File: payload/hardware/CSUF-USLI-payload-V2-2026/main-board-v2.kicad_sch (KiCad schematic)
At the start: 29 parts, among them J1 Servo JST, J10 8.4V IN, J11 Chassis Input, J12 Servo VCC, J13 Servo GND, J14 11.1V IN, J15 8.4V RESERVE, J16 11.1V RESERVE, J17 Driver Input, J2 Drill x 11.1V OUT, J4 BTS7960 Output, J6 Reserve JST, J9 Soil Sensor Power, Q3 IRLZ44N, U1 DEV-16771, U2 Adafruit BMP280, U3 RYLR896, U4 RYLR896, U5 Modbus to UART

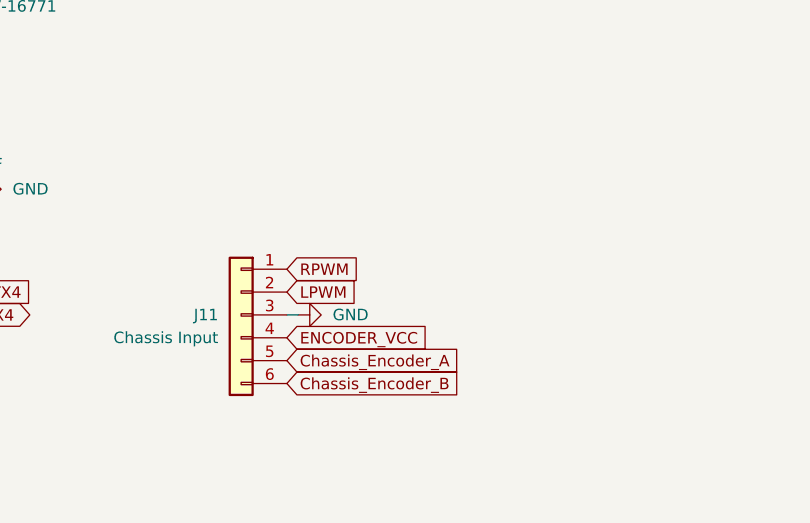
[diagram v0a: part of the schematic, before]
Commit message: trying to route traces
bad bad bad
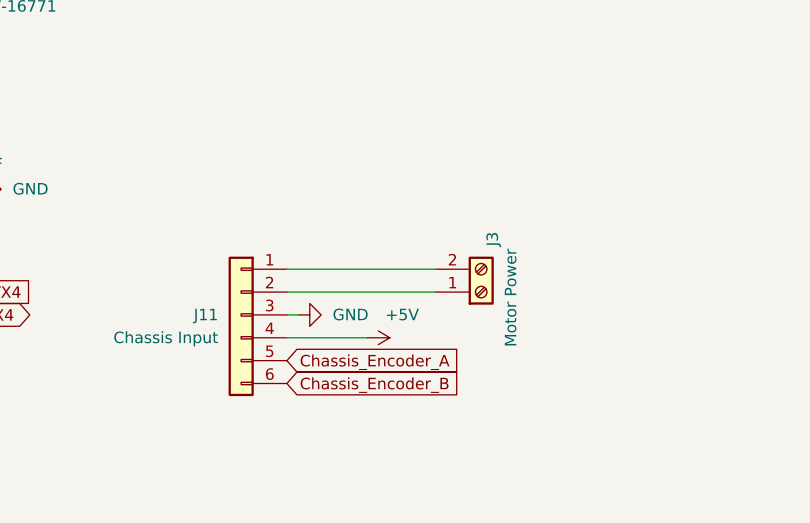
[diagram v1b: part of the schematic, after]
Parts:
- added J3: Motor Power, Phoenix_Screw_Connectors:Edit_TerminalBlock_Phoenix_MKDS-1,5-2_1x02_P5.00mm_Horizontal, symbol Connector:Screw_Terminal_01x02
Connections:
- net ENCODER_VCC is gone; now on net +5V: J11.4 (Pin_4)
- net LPWM: no longer J11.2 (Pin_2)
- net RPWM: no longer J11.1 (Pin_1)
- new net: J11.1 (Pin_1), J3.2 (Pin_2)
- new net: J11.2 (Pin_2), J3.1 (Pin_1)
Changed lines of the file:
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@@
 	(wire
 		(pts
+			(xy 139.7 161.29) (xy 156.21 161.29)
+		)
+		(stroke
+			(width 0)
+			(type default)
+		)
+	)
+	(wire
+		(pts
 			(xy 96.52 151.13) (xy 96.52 152.4)
 		)
@@
 	(wire
 		(pts
+			(xy 139.7 163.83) (xy 156.21 163.83)
+		)
+		(stroke
+			(width 0)
+			(type default)
+		)
+	)
+	(wire
+		(pts
 			(xy 181.61 29.21) (xy 181.61 38.1)
 		)
@@
 	(wire
 		(pts
+			(xy 139.7 168.91) (xy 148.59 168.91)
+		)
+		(stroke
+			(width 0)
+			(type default)
+		)
+	)
+	(wire
+		(pts
 			(xy 139.7 166.37) (xy 140.97 166.37)
 		)
@@
 		)
 	)
-	(global_label "LPWM"
-		(shape input)
-		(at 139.7 163.83 0)
-		(fields_autoplaced yes)
-		(effects
-			(font
-				(size 1.27 1.27)
-			)
-			(justify left)
-		)
-		(property "Intersheetrefs" "${INTERSHEET_REFS}"
-			(at 147.8861 163.83 0)
-			(effects
-				(font
-					(size 1.27 1.27)
-				)
-				(justify left)
-				(hide yes)
-			)
-		)
-	)
 	(global_label "SCL"
 		(shape output)
@@
 		)
 	)
-	(global_label "ENCODER_VCC"
-		(shape input)
-		(at 139.7 168.91 0)
-		(fields_autoplaced yes)
-		(effects
-			(font
-				(size 1.27 1.27)
-			)
-			(justify left)
-		)
-		(property "Intersheetrefs" "${INTERSHEET_REFS}"
-			(at 156.0504 168.91 0)
-			(effects
-				(font
-					(size 1.27 1.27)
-				)
-				(justify left)
-				(hide yes)
-			)
-		)
-	)
 	(global_label "RESERVE_3"
 		(shape input)
@@
 		)
 	)
-	(global_label "RPWM"
-		(shape input)
-		(at 139.7 161.29 0)
-		(fields_autoplaced yes)
-		(effects
-			(font
-				(size 1.27 1.27)
-			)
-			(justify left)
-		)
-		(property "Intersheetrefs" "${INTERSHEET_REFS}"
-			(at 148.128 161.29 0)
-			(effects
-				(font
-					(size 1.27 1.27)
-				)
-				(justify left)
-				(hide yes)
-			)
-		)
-	)
 	(global_label "SERVO_2"
 		(shape input)
@@
 	)
 	(symbol
+		(lib_id "Connector:Screw_Terminal_01x02")
+		(at 161.29 163.83 0)
+		(mirror x)
+		(unit 1)
+		(exclude_from_sim no)
+		(in_bom yes)
+		(on_board yes)
+		(dnp no)
+		(property "Reference" "J3"
+			(at 162.5601 158.75 90)
+			(effects
+				(font
+					(size 1.27 1.27)
+				)
+				(justify right)
+			)
+		)
+		(property "Value" "Motor Power"
+			(at 164.592 169.926 90)
+			(effects
+				(font
+					(size 1.27 1.27)
+				)
+				(justify right)
+			)
+		)
+		(property "Footprint" "Phoenix_Screw_Connectors:Edit_TerminalBlock_Phoenix_MKDS-1,5-2_1x02_P5.00mm_Horizontal"
+			(at 161.29 163.83 0)
+			(effects
+				(font
+					(size 1.27 1.27)
+				)
+				(hide yes)
+			)
+		)
+		(property "Datasheet" "~"
+			(at 161.29 163.83 0)
+			(effects
+				(font
+					(size 1.27 1.27)
+				)
+				(hide yes)
+			)
+		)
+		(property "Description" "Generic screw terminal, single row, 01x02, script generated (kicad-library-utils/schlib/autogen/connector/)"
+			(at 161.29 163.83 0)
+			(effects
+				(font
+					(size 1.27 1.27)
+				)
+				(hide yes)
+			)
+		)
+		(pin "1"
+		)
+		(pin "2"
+		)
+		(instances
+			(project "main-board-v2"
+				(path "/2777fc69-937c-438e-abe9-028d5203e7d8"
+					(reference "J3")
+					(unit 1)
+				)
+			)
+		)
+	)
+	(symbol
 		(lib_id "power:+3V3")
 		(at 64.77 151.13 0)
@@
 					(unit 1)
 				)
+			)
+		)
+	)
+	(symbol
+		(lib_id "power:+8V")
+		(at 148.59 168.91 270)
+		(unit 1)
+		(exclude_from_sim no)
+		(in_bom yes)
+		(on_board yes)
+		(dnp no)
+		(property "Reference" "#PWR017"
+			(at 144.78 168.91 0)
+			(effects
+				(font
+					(size 1.27 1.27)
+				)
+				(hide yes)
+			)
+		)
+		(property "Value" "+5V"
+			(at 150.622 166.37 90)
+			(effects
+				(font
+					(size 1.27 1.27)
+				)
+				(justify left)
+			)
+		)
+		(property "Footprint" ""
+			(at 148.59 168.91 0)
+			(effects
+				(font
+					(size 1.27 1.27)
+				)
+				(hide yes)
+			)
+		)
+		(property "Datasheet" ""
+			(at 148.59 168.91 0)
+			(effects
+				(font
+					(size 1.27 1.27)
+				)
+				(hide yes)
+			)
+		)
+		(property "Description" "Power symbol creates a global label with name \"+8V\""
+			(at 148.59 168.91 0)
+			(effects
+				(font
+					(size 1.27 1.27)
+				)
+				(hide yes)
+			)
+		)
+		(pin "1"
+		)
+		(instances
+			(project "main-board-v2"
+				(path "/2777fc69-937c-438e-abe9-028d5203e7d8"
+					(reference "#PWR017")
+					(unit 1)
+				)
